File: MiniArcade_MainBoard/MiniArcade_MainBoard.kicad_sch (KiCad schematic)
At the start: 31 parts, among them J1 62701021721, J2 Conn_01x05_Pin, J3 Conn_01x06_Pin, J4 F3311A7H121026E200, SW1 EVPAA, U1 ATSAMD21J18A-A, U2 LM321

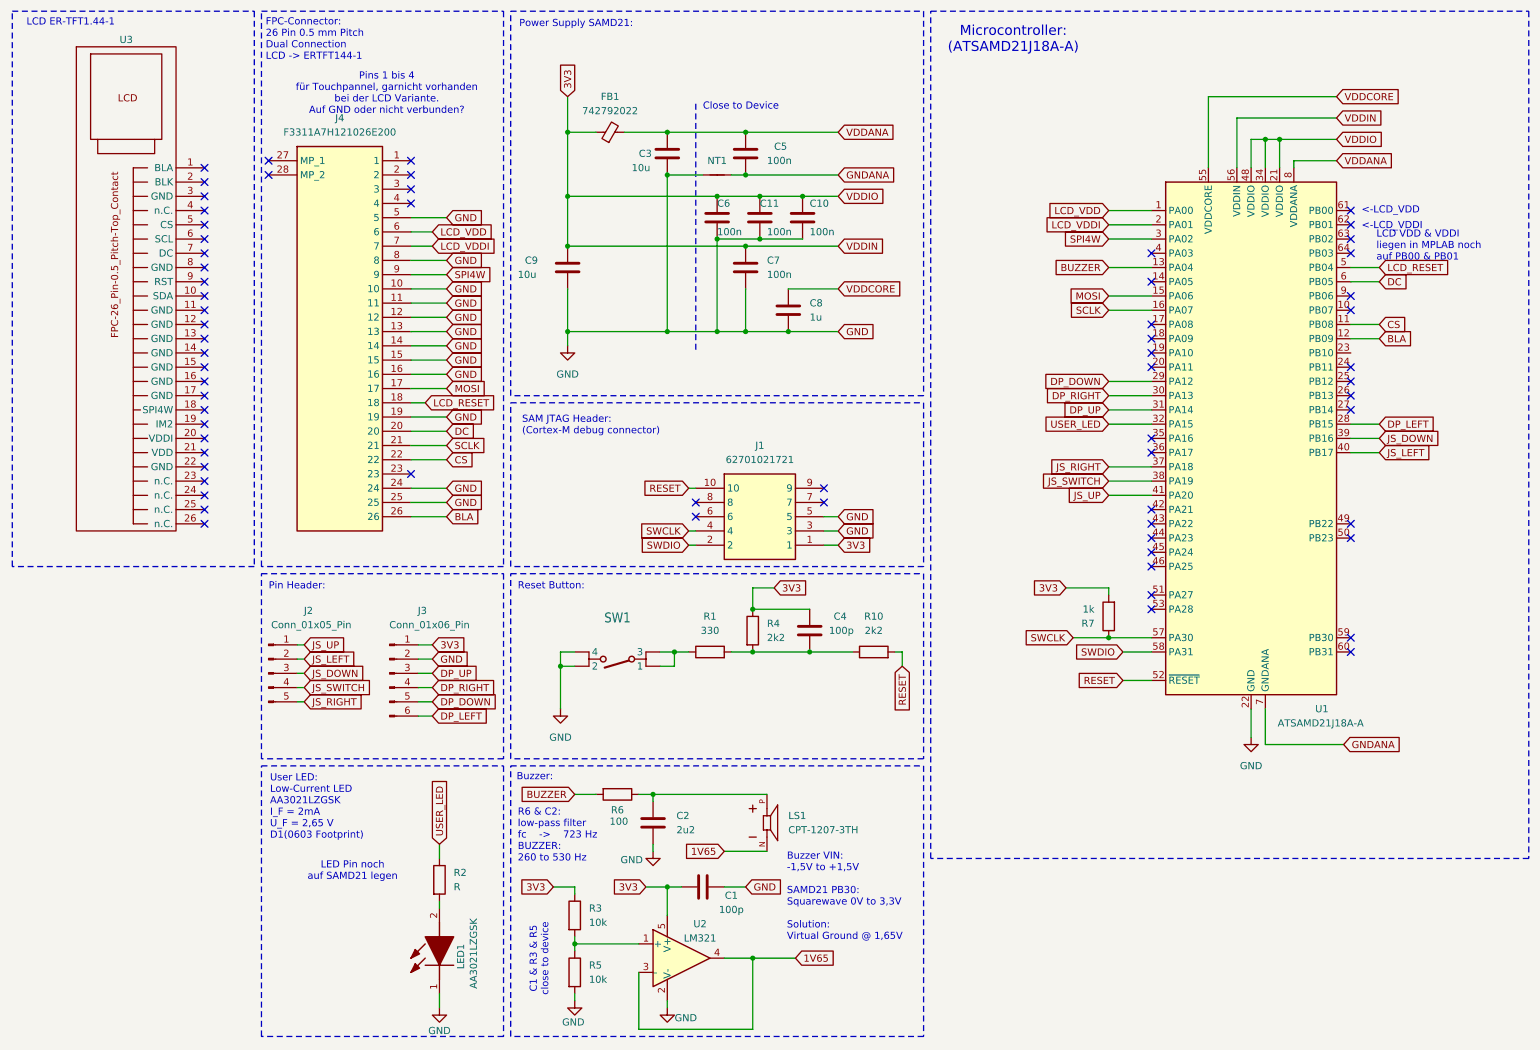
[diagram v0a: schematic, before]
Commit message: 17 11 2025
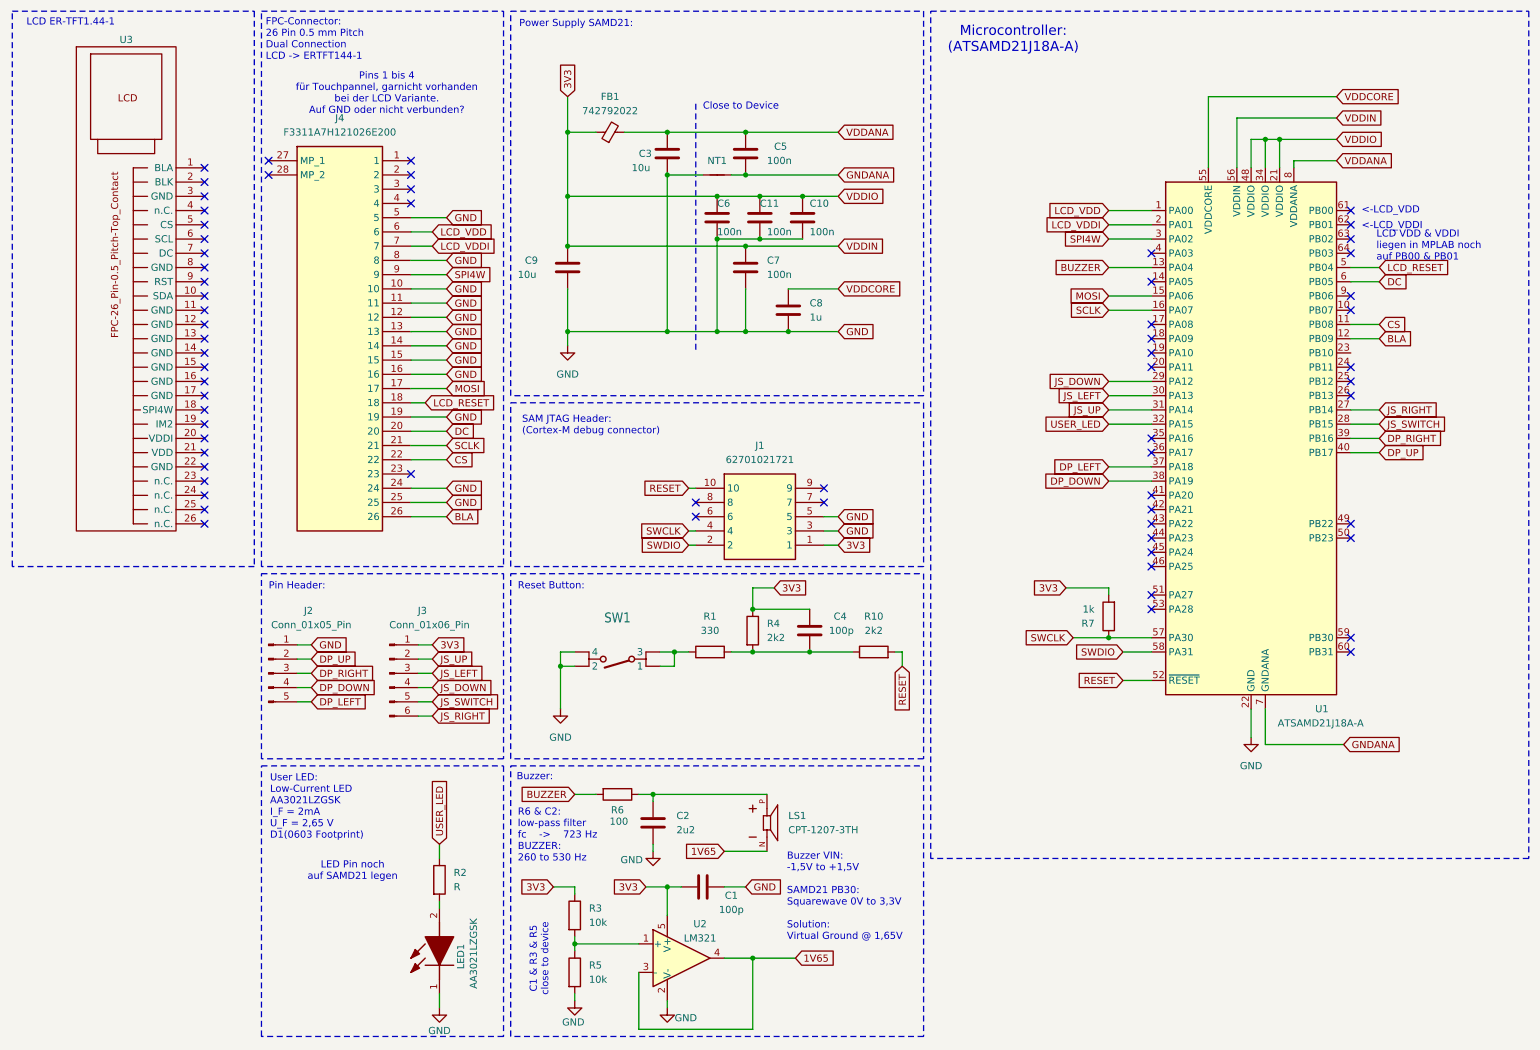
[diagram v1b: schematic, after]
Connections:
- net DP_DOWN: now also J2.4 (Pin_4), U1.38 (PA19); no longer J3.5 (Pin_5), U1.29 (PA12)
- net DP_LEFT: now also J2.5 (Pin_5), U1.37 (PA18); no longer J3.6 (Pin_6), U1.28 (PB15)
- net DP_RIGHT: now also J2.3 (Pin_3), U1.39 (PB16); no longer J3.4 (Pin_4), U1.30 (PA13)
- net DP_UP: now also J2.2 (Pin_2), U1.40 (PB17); no longer J3.3 (Pin_3), U1.31 (PA14)
- net GND: now also J2.1 (Pin_1); no longer J3.2 (Pin_2)
- net JS_DOWN: now also J3.4 (Pin_4), U1.29 (PA12); no longer J2.3 (Pin_3), U1.39 (PB16)
- net JS_LEFT: now also J3.3 (Pin_3), U1.30 (PA13); no longer J2.2 (Pin_2), U1.40 (PB17)
- net JS_RIGHT: now also J3.6 (Pin_6), U1.27 (PB14); no longer J2.5 (Pin_5), U1.37 (PA18)
- net JS_SWITCH: now also J3.5 (Pin_5), U1.28 (PB15); no longer J2.4 (Pin_4), U1.38 (PA19)
- net JS_UP: now also J3.2 (Pin_2), U1.31 (PA14); no longer J2.1 (Pin_1), U1.41 (PA20)
